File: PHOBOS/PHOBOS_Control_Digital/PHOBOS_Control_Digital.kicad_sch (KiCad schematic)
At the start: 73 parts, among them J12 PWR, J14 PS1-2, J15 PS3-4, J2 RF_OUT, J3 USB4056-03-A_REVA2, J4 Screw_Terminal_01x02, J8 BOOT, U1 SX1280IMLTRT, U2 W25Q128JVSIQ, U3 NCP1117-3.3_SOT223, U4 RP2040, U5 TPS60403DBV, Y1 C1E-52.000-10-1012-X-M, Y2 ABM8-272-T3

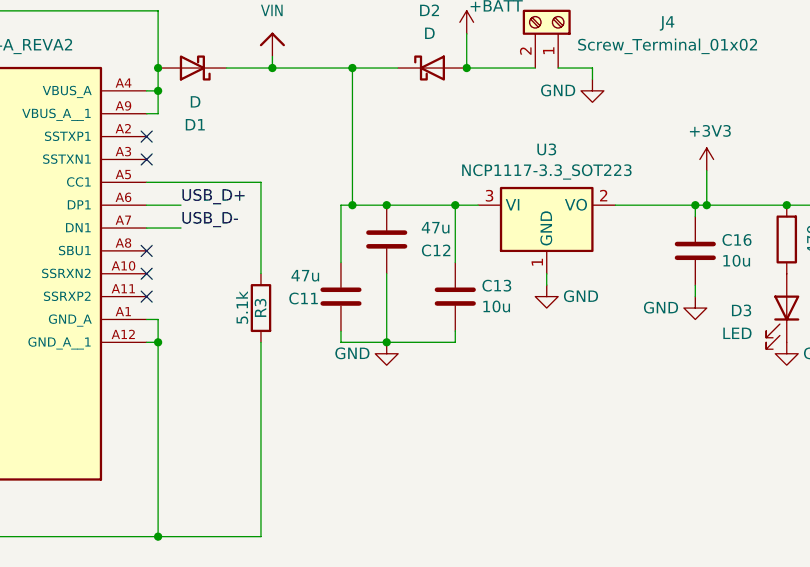
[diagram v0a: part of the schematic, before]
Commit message: BOM Updated
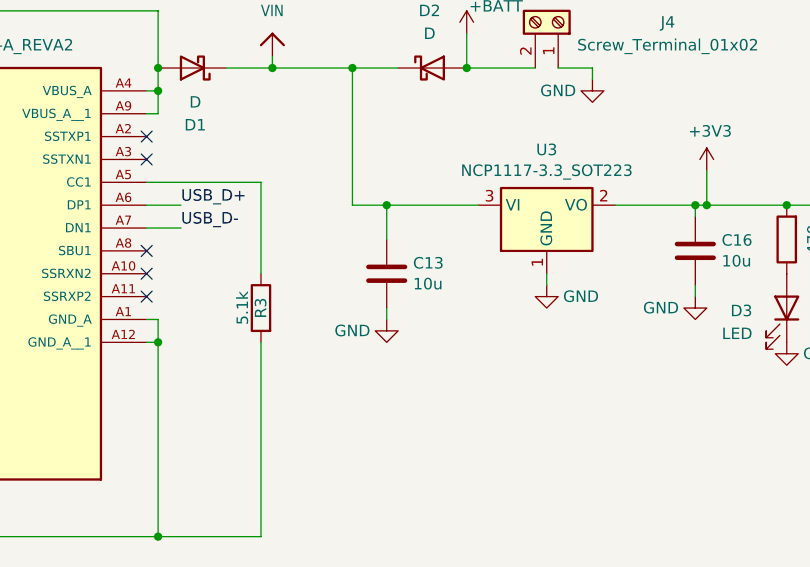
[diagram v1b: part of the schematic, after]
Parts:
- removed C11: 47u, Capacitor_SMD:C_0805_2012Metric_Pad1.18x1.45mm_HandSolder, symbol Device:C
- removed C12: 47u, Capacitor_SMD:C_1206_3216Metric, symbol Device:C
- C13, C16, C17: MFG # (none) -> CL10X106MO8NRNC
- C14, C15: MFG # (none) -> GJM1555C1H150GB01D
- C18, C19, C21, C23, C24, C25, C30, C31, C36, C7: MFG # (none) -> CL05B104KO5NNNC
- C20, C22, C37, C38, C39: MFG # (none) -> C0603X5R500-105KNP-CT
- D1, D2: MFG # (none) -> CD0603-B0340R
- D3: MFG # (none) -> QBLP601-IB5-S2897
- J12: MFG # (none) -> SM06B-GHS-TB
- J14, J15: MFG # (none) -> SM10B-GHS-TB
- J3: MFG # (none) -> USB4056-03-A
- J4: MFG # (none) -> OSTTE020104
- R1, R3: MFG # (none) -> AC0402FR-7W5K1L
- R13, R19: MFG # (none) -> AC0402FR-7W4K7L
- R14: MFG # (none) -> CRGCQ0402F330K
- R16: MFG # (none) -> AC0402FR-7W100KL
- R4: MFG # (none) -> AC0402FR-7W470RL
- R5: MFG # (none) -> AC0402FR-7W1KL
- R6: MFG # (none) -> AC0402FR-7W10KL
- R7, R8: MFG # (none) -> RC0402FR-7W27RL
- U2: MFG # (none) -> W25Q128JVSIQ
- U3: MFG # (none) -> NCP1117ST33T3G
- U4: MFG # (none) -> SC0914(13)
- U5: MFG # (none) -> TPS60403DBV
- Y2: MFG # (none) -> ABM8-272-T3
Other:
- moved on the sheet: C13
